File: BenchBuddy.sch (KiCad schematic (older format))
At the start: 0 parts

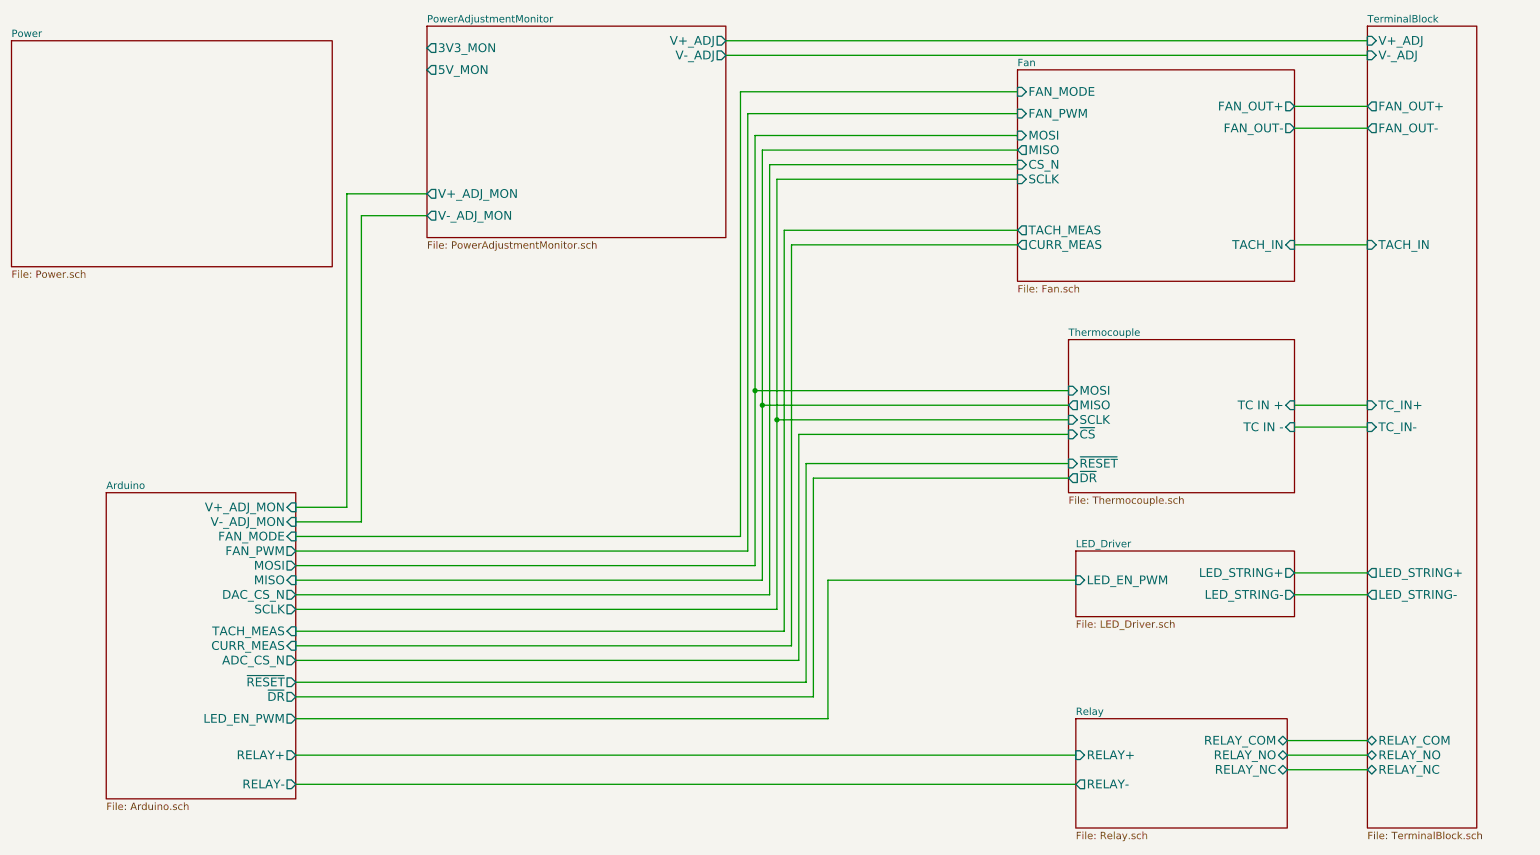
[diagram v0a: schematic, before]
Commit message: Power Modification Module
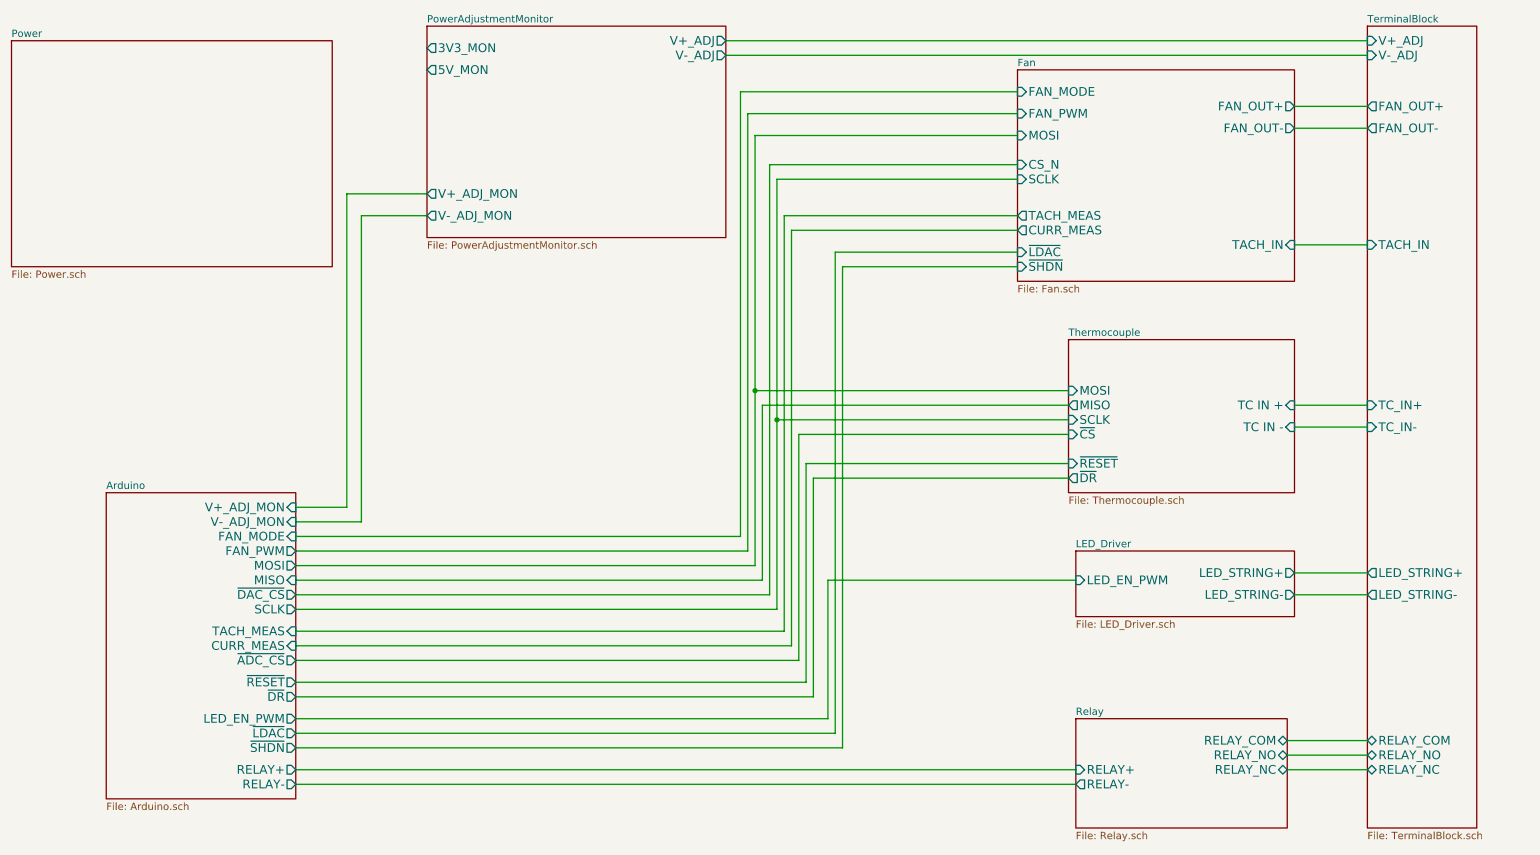
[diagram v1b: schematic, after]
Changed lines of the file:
@@
 Sheet 1 9
 Title ""
-Date "17 oct 2013"
+Date "27 oct 2013"
 Rev ""
 Comp ""
@@
 F1 "Fan.sch" 50
 F2 "MOSI" I L 7850 1550 60
-F3 "MISO" O L 7850 1650 60
-F4 "CS_N" I L 7850 1750 60
-F5 "SCLK" I L 7850 1850 60
-F6 "TACH_MEAS" O L 7850 2200 60
-F7 "FAN_OUT+" O R 9750 1350 60
-F8 "FAN_OUT-" O R 9750 1500 60
-F9 "TACH_IN" I R 9750 2300 60
-F10 "CURR_MEAS" O L 7850 2300 60
-F11 "FAN_PWM" I L 7850 1400 60
-F12 "FAN_MODE" I L 7850 1250 60
+F3 "CS_N" I L 7850 1750 60
+F4 "SCLK" I L 7850 1850 60
+F5 "TACH_MEAS" O L 7850 2100 60
+F6 "FAN_OUT+" O R 9750 1350 60
+F7 "FAN_OUT-" O R 9750 1500 60
+F8 "TACH_IN" I R 9750 2300 60
+F9 "CURR_MEAS" O L 7850 2200 60
+F10 "FAN_PWM" I L 7850 1400 60
+F11 "FAN_MODE" I L 7850 1250 60
+F12 "~LDAC" I L 7850 2350 60
+F13 "~SHDN" I L 7850 2450 60
 $EndSheet
 $Sheet
@@
 F0 "Relay" 50
 F1 "Relay.sch" 50
-F2 "RELAY+" I L 8250 5800 60
+F2 "RELAY+" I L 8250 5900 60
 F3 "RELAY-" O L 8250 6000 60
 F4 "RELAY_NC" B R 9700 5900 60
@@
 	6050 4500 2900 4500
 Wire Wire Line
-	6100 4600 2900 4600
-Wire Wire Line
-	6100 1650 6100 4600
-Wire Wire Line
-	6100 1650 7850 1650
-Wire Wire Line
 	7850 1750 6150 1750
 Wire Wire Line
@@
 	6200 1850 7850 1850
 Wire Wire Line
-	7850 2200 6250 2200
-Wire Wire Line
-	6250 2200 6250 4950
+	7850 2100 6250 2100
+Wire Wire Line
+	6250 2100 6250 4950
 Wire Wire Line
 	6250 4950 2900 4950
@@
 	2900 5050 6300 5050
 Wire Wire Line
-	6300 5050 6300 2300
-Wire Wire Line
-	6300 2300 7850 2300
+	6300 5050 6300 2200
+Wire Wire Line
+	6300 2200 7850 2200
 Wire Wire Line
 	8200 3300 6050 3300
@@
 Wire Wire Line
 	8200 3400 6100 3400
-Connection ~ 6100 3400
 $Sheet
 S 1600 4000 1300 2100
@@
 F5 "SCLK" O R 2900 4800 60
 F6 "CURR_MEAS" I R 2900 5050 60
-F7 "RELAY+" O R 2900 5800 60
+F7 "RELAY+" O R 2900 5900 60
 F8 "RELAY-" O R 2900 6000 60
 F9 "V+_ADJ_MON" I R 2900 4100 60
 F10 "V-_ADJ_MON" I R 2900 4200 60
 F11 "LED_EN_PWM" O R 2900 5550 60
-F12 "DAC_CS_N" O R 2900 4700 60
-F13 "ADC_CS_N" O R 2900 5150 60
-F14 "FAN_PWM" O R 2900 4400 60
-F15 "FAN_MODE" I R 2900 4300 60
-F16 "~RESET" O R 2900 5300 60
-F17 "~DR" O R 2900 5400 60
+F12 "FAN_PWM" O R 2900 4400 60
+F13 "FAN_MODE" I R 2900 4300 60
+F14 "~RESET" O R 2900 5300 60
+F15 "~DR" O R 2900 5400 60
+F16 "~LDAC" O R 2900 5650 60
+F17 "~SHDN" O R 2900 5750 60
+F18 "~DAC_CS" O R 2900 4700 60
+F19 "~ADC_CS" O R 2900 5150 60
 $EndSheet
 Wire Wire Line
@@
 	6550 4600 8250 4600
 Wire Wire Line
-	2900 5800 8250 5800
+	2900 5900 8250 5900
 Wire Wire Line
 	8250 6000 2900 6000
@@
 Wire Wire Line
 	6450 5400 2900 5400
+Wire Wire Line
+	6100 3400 6100 4600
+Wire Wire Line
+	6100 4600 2900 4600
+Wire Wire Line
+	2900 5650 6600 5650
+Wire Wire Line
+	6600 5650 6600 2350
+Wire Wire Line
+	6600 2350 7850 2350
+Wire Wire Line
+	7850 2450 6650 2450
+Wire Wire Line
+	6650 2450 6650 5750
+Wire Wire Line
+	6650 5750 2900 5750
 $EndSCHEMATC
